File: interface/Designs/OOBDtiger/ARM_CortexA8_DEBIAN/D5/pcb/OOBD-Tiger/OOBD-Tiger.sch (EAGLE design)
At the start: 88 parts, among them IC3 DS1307, IC4 DS3231, Q2 32.768kHz, U1 SY6280, U10 MP1482DS, U2 SN65HVD230(SO8), U6 SN65HVD230(SO8)

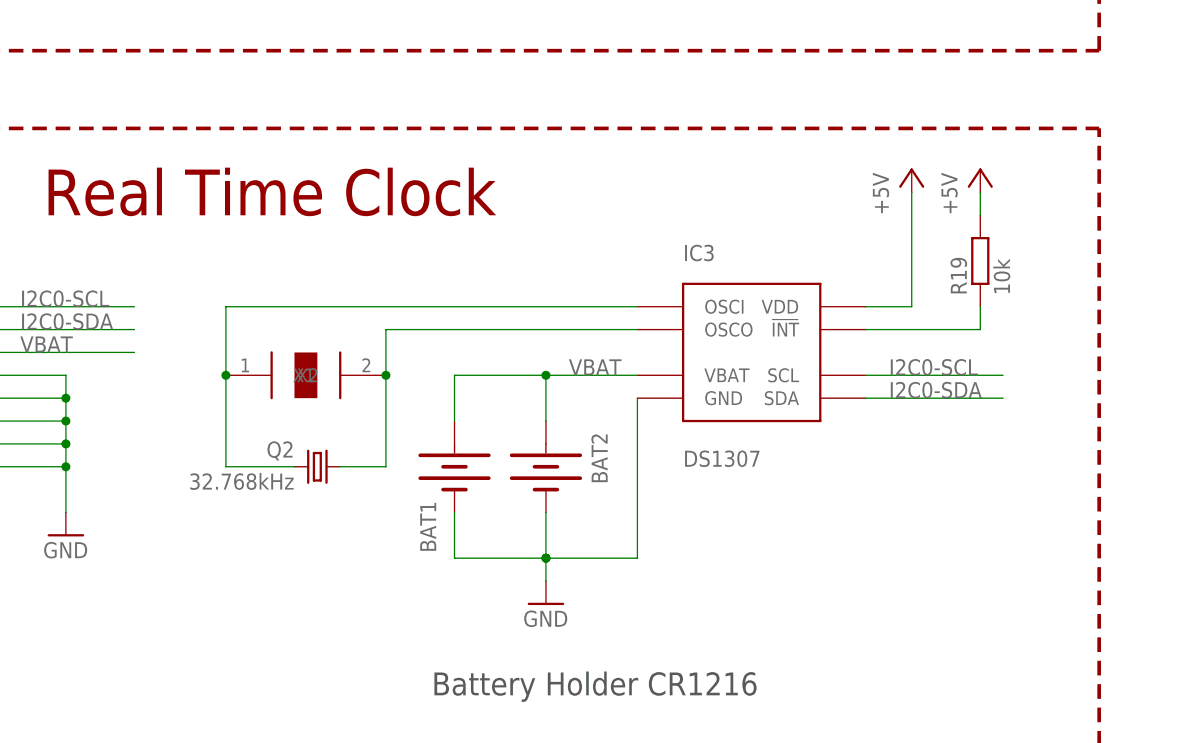
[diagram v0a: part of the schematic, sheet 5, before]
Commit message: Aufgeräumt mit Mike
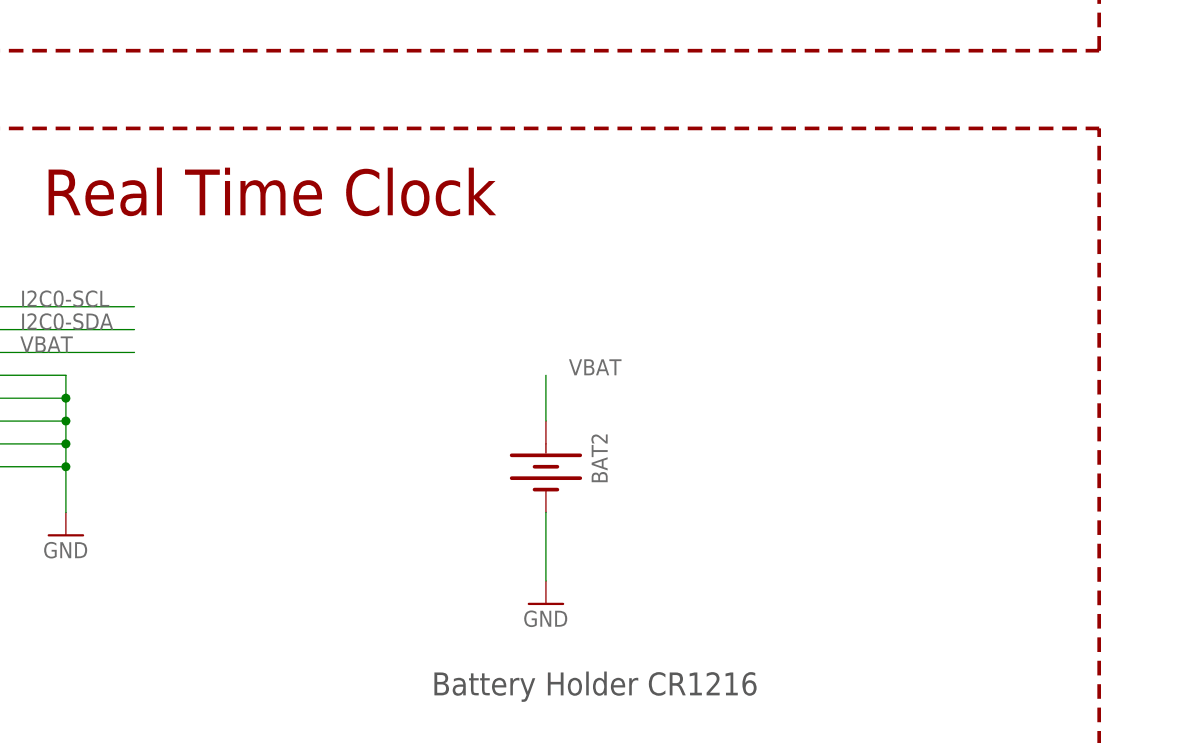
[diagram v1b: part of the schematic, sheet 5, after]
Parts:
- removed BAT1: (no value), SparkFun:BATTERY12MM
- removed IC3: DS1307, PierpaoloSmartSpaceSolutions:PCF8523SOIC8
- removed Q2: 32.768kHz, crystal:CRYSTALTC26H
- removed R19: 10k, rcl:R-EU_R0603
- removed U$3: XTAL32K, PierpaoloSmartSpaceSolutions:XTAL32K
- C1, C47: device rcl:C-EU025-024X044 -> rcl:C-EU2
- R7: device rcl:R-EU_0204/2V -> rcl:R-EU_R0603
- USB_HOST2: device OLIMEX_CONNECTORS:USB_SHIELDUSB_A_VERTICAL -> OLIMEX_CONNECTORS:USB_SHIELD1
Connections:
- removed net N$3: IC3.!INT, R19.1
- removed net OSCI: IC3.OSCI, Q2.2, U$3.X1
- removed net OSCO: IC3.OSCO, Q2.1, U$3.X2
- net +5V: no longer IC3.VDD, R19.2
- net GND: no longer BAT1.-, IC3.GND
- net I2C0-SCL: no longer IC3.SCL
- net I2C0-SDA: no longer IC3.SDA
- net VBAT: no longer BAT1.+, IC3.VBAT
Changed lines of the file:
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@@
 <?xml version="1.0" encoding="utf-8"?>
 <!DOCTYPE eagle SYSTEM "eagle.dtd">
-<eagle version="6.4">
+<eagle version="7.6.0">
 <drawing>
 <settings>
@@
 <part name="R41" library="rcl" deviceset="R-EU_" device="0204/2V" value="10k"/>
 <part name="V52" library="supply2" deviceset="VCC" device="" value="3.3V"/>
-<part name="C47" library="rcl" deviceset="C-EU" device="025-024X044" value="100nF"/>
+<part name="C47" library="rcl" deviceset="C-EU" device="2" value="100nF"/>
 <part name="GND98" library="supply1" deviceset="GND" device="" value=""/>
 <part name="R42" library="rcl" deviceset="R-EU_" device="0204/2V" value="120R"/>
@@
 <part name="R5" library="rcl" deviceset="R-EU_" device="0204/2V" value="10k"/>
 <part name="V2" library="supply2" deviceset="VCC" device="" value="3.3V"/>
-<part name="C1" library="rcl" deviceset="C-EU" device="025-024X044" value="100nF"/>
+<part name="C1" library="rcl" deviceset="C-EU" device="2" value="100nF"/>
 <part name="GND5" library="supply1" deviceset="GND" device="" value=""/>
 <part name="R6" library="rcl" deviceset="R-EU_" device="0204/2V" value="120R"/>
-<part name="R7" library="rcl" deviceset="R-EU_" device="0204/2V" value="NA"/>
+<part name="R7" library="rcl" deviceset="R-EU_" device="R0603" value="NA"/>
 <part name="OBD2-CONNECTOR" library="pinhead" deviceset="PINHD-2X5" device="/90"/>
 <part name="R8" library="resistor" deviceset="R-EU_" device="R0603" value="10K">
@@
 <part name="P+2" library="supply1" deviceset="+12V" device=""/>
 <part name="P+4" library="supply1" deviceset="+12V" device=""/>
-<part name="U$3" library="PierpaoloSmartSpaceSolutions" deviceset="XTAL32K" device=""/>
-<part name="Q2" library="crystal" deviceset="CRYSTAL" device="TC26H" value="32.768kHz"/>
 <part name="GND7" library="supply1" deviceset="GND" device=""/>
-<part name="IC3" library="PierpaoloSmartSpaceSolutions" deviceset="PCF8523" device="SOIC8" value="DS1307"/>
 <part name="GND33" library="supply1" deviceset="GND" device=""/>
 <part name="C9" library="rcl" deviceset="C-EU" device="C0603" value="1uF"/>
-<part name="R19" library="rcl" deviceset="R-EU_" device="R0603" value="10k"/>
-<part name="BAT1" library="SparkFun" deviceset="BATTERY" device="12MM"/>
-<part name="P+14" library="supply1" deviceset="+5V" device=""/>
 <part name="IC4" library="DS3231_industrialberry" deviceset="DS3231" device="SOIC-16W" value="DS3231"/>
 <part name="GND11" library="supply1" deviceset="GND" device=""/>
 <part name="GND16" library="supply1" deviceset="GND" device=""/>
 <part name="BAT2" library="SparkFun" deviceset="BATTERY" device="12PTH"/>
-<part name="USB_HOST2" library="OLIMEX_CONNECTORS" deviceset="USB_SHIELD" device="USB_A_VERTICAL" value="USB_A_VERTICAL"/>
+<part name="USB_HOST2" library="OLIMEX_CONNECTORS" deviceset="USB_SHIELD" device="1" value="USB_A_VERTICAL"/>
 <part name="L5" library="rcl" deviceset="L-US" device="L0805_5MIL_DWS" value="FB0805/600R/2A"/>
 <part name="C3" library="rcl" deviceset="C-EU" device="C0603_DWS" value="100nF"/>
@@
 <part name="+3V2" library="supply1" deviceset="+3V3" device=""/>
 <part name="R20" library="rcl" deviceset="R-EU_" device="R0603" value="10k"/>
-<part name="P+6" library="supply1" deviceset="+5V" device=""/>
 <part name="+3V3" library="supply1" deviceset="+3V3" device=""/>
 <part name="+3V4" library="supply1" deviceset="+3V3" device=""/>
@@
 <instance part="GND26" gate="1" x="157.48" y="96.52"/>
 <instance part="P+4" gate="1" x="17.78" y="154.94"/>
-<instance part="U$3" gate="G$1" x="96.52" y="53.34" rot="MR180"/>
-<instance part="Q2" gate="G$1" x="99.06" y="43.18" rot="MR0"/>
 <instance part="GND7" gate="1" x="124.46" y="27.94"/>
-<instance part="IC3" gate="G$1" x="147.32" y="55.88"/>
 <instance part="GND33" gate="1" x="20.32" y="35.56"/>
 <instance part="C9" gate="G$1" x="20.32" y="45.72" rot="R180"/>
-<instance part="R19" gate="G$1" x="172.72" y="66.04" rot="R90"/>
-<instance part="BAT1" gate="G$1" x="114.3" y="43.18" smashed="yes" rot="R270">
-<attribute name="NAME" x="110.49" y="39.37" size="1.778" layer="95" rot="R270"/>
-<attribute name="VALUE" x="107.95" y="46.99" size="1.778" layer="96" rot="R270"/>
-</instance>
-<instance part="P+14" gate="1" x="165.1" y="76.2"/>
 <instance part="IC4" gate="G$1" x="50.8" y="50.8"/>
 <instance part="GND11" gate="1" x="71.12" y="35.56"/>
@@
 <instance part="+3V2" gate="G$1" x="35.56" y="73.66"/>
 <instance part="R20" gate="G$1" x="27.94" y="63.5" rot="R90"/>
-<instance part="P+6" gate="1" x="172.72" y="76.2"/>
 <instance part="+3V3" gate="G$1" x="27.94" y="73.66"/>
 </instances>
@@
 </segment>
 <segment>
-<wire x1="124.46" y1="33.02" x2="124.46" y2="30.48" width="0.1524" layer="91"/>
-<wire x1="124.46" y1="33.02" x2="134.62" y2="33.02" width="0.1524" layer="91"/>
-<wire x1="134.62" y1="33.02" x2="134.62" y2="50.8" width="0.1524" layer="91"/>
-<junction x="124.46" y="33.02"/>
 <pinref part="GND7" gate="1" pin="GND"/>
-<pinref part="IC3" gate="G$1" pin="GND"/>
-<pinref part="BAT1" gate="G$1" pin="-"/>
 <pinref part="BAT2" gate="G$1" pin="-"/>
-<wire x1="124.46" y1="38.1" x2="124.46" y2="33.02" width="0.1524" layer="91"/>
-<wire x1="124.46" y1="33.02" x2="114.3" y2="33.02" width="0.1524" layer="91"/>
-<wire x1="114.3" y1="33.02" x2="114.3" y2="38.1" width="0.1524" layer="91"/>
-<junction x="124.46" y="33.02"/>
+<wire x1="124.46" y1="38.1" x2="124.46" y2="30.48" width="0.1524" layer="91"/>
 </segment>
 <segment>
@@
 <pinref part="P+5" gate="1" pin="+5V"/>
 <pinref part="R86" gate="G$1" pin="1"/>
-</segment>
-<segment>
-<wire x1="165.1" y1="60.96" x2="165.1" y2="73.66" width="0.1524" layer="91"/>
-<wire x1="160.02" y1="60.96" x2="165.1" y2="60.96" width="0.1524" layer="91"/>
-<pinref part="IC3" gate="G$1" pin="VDD"/>
-<pinref part="P+14" gate="1" pin="+5V"/>
-</segment>
-<segment>
-<wire x1="172.72" y1="73.66" x2="172.72" y2="71.12" width="0.1524" layer="91"/>
-<pinref part="R19" gate="G$1" pin="2"/>
-<pinref part="P+6" gate="1" pin="+5V"/>
 </segment>
 </net>
@@
 <net name="I2C0-SDA" class="0">
 <segment>
-<wire x1="175.26" y1="50.8" x2="160.02" y2="50.8" width="0.1524" layer="91"/>
-<label x="162.56" y="50.8" size="1.778" layer="95"/>
-<pinref part="IC3" gate="G$1" pin="SDA"/>
-</segment>
-<segment>
 <wire x1="78.74" y1="58.42" x2="63.5" y2="58.42" width="0.1524" layer="91"/>
 <label x="66.04" y="58.42" size="1.778" layer="95"/>
@@
 <net name="I2C0-SCL" class="0">
 <segment>
-<wire x1="175.26" y1="53.34" x2="160.02" y2="53.34" width="0.1524" layer="91"/>
-<label x="162.56" y="53.34" size="1.778" layer="95"/>
-<pinref part="IC3" gate="G$1" pin="SCL"/>
-</segment>
-<segment>
 <wire x1="78.74" y1="60.96" x2="63.5" y2="60.96" width="0.1524" layer="91"/>
 <label x="66.04" y="60.96" size="1.778" layer="95"/>
@@
 </segment>
 </net>
-<net name="N$3" class="0">
-<segment>
-<wire x1="160.02" y1="58.42" x2="172.72" y2="58.42" width="0.1524" layer="91"/>
-<wire x1="172.72" y1="58.42" x2="172.72" y2="60.96" width="0.1524" layer="91"/>
-<pinref part="IC3" gate="G$1" pin="!INT"/>
-<pinref part="R19" gate="G$1" pin="1"/>
-</segment>
-</net>
 <net name="VBAT" class="0">
 <segment>
@@
 </segment>
 <segment>
-<pinref part="BAT1" gate="G$1" pin="+"/>
-<wire x1="114.3" y1="48.26" x2="114.3" y2="53.34" width="0.1524" layer="91"/>
-<pinref part="IC3" gate="G$1" pin="VBAT"/>
-<wire x1="114.3" y1="53.34" x2="124.46" y2="53.34" width="0.1524" layer="91"/>
 <pinref part="BAT2" gate="G$1" pin="+"/>
-<wire x1="124.46" y1="53.34" x2="134.62" y2="53.34" width="0.1524" layer="91"/>
 <wire x1="124.46" y1="48.26" x2="124.46" y2="53.34" width="0.1524" layer="91"/>
-<junction x="124.46" y="53.34"/>
 <label x="127" y="53.34" size="1.778" layer="95"/>
 </segment>
 </net>
-<net name="OSCI" class="0">
-<segment>
-<wire x1="96.52" y1="43.18" x2="88.9" y2="43.18" width="0.1524" layer="91"/>
-<wire x1="88.9" y1="43.18" x2="88.9" y2="53.34" width="0.1524" layer="91"/>
-<wire x1="88.9" y1="53.34" x2="88.9" y2="60.96" width="0.1524" layer="91"/>
-<junction x="88.9" y="53.34"/>
-<pinref part="Q2" gate="G$1" pin="2"/>
-<pinref part="U$3" gate="G$1" pin="X1"/>
-<wire x1="88.9" y1="60.96" x2="134.62" y2="60.96" width="0.1524" layer="91"/>
-<pinref part="IC3" gate="G$1" pin="OSCI"/>
-</segment>
-</net>
-<net name="OSCO" class="0">
-<segment>
-<wire x1="101.6" y1="43.18" x2="106.68" y2="43.18" width="0.1524" layer="91"/>
-<wire x1="106.68" y1="43.18" x2="106.68" y2="53.34" width="0.1524" layer="91"/>
-<wire x1="106.68" y1="53.34" x2="106.68" y2="58.42" width="0.1524" layer="91"/>
-<junction x="106.68" y="53.34"/>
-<pinref part="Q2" gate="G$1" pin="1"/>
-<pinref part="U$3" gate="G$1" pin="X2"/>
-<pinref part="IC3" gate="G$1" pin="OSCO"/>
-<wire x1="134.62" y1="58.42" x2="106.68" y2="58.42" width="0.1524" layer="91"/>
-</segment>
-</net>
